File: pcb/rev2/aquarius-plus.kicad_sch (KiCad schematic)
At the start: 216 parts, among them J1 Cassette in, J10 Audio out, J11 Hand controller 2, J12 ESP USB Host, J13 Power in, J14 FPGA spare, J15 Expansion port, J16 ESP32 spare, J2 Cassette out, J3 Amphenol GSD090012SEU, J4 Printer, J5 Hand controller 1, J6 VGA, J7 DBG, J8 USB_A, J9 USB_A, Q1 BC847C, Q2 BC847C, SW1 SW_DPDT_x2, U1 XC3S200-4TQG144, U10 IS61C5128AS-25QLI, U11 74LVC4245APW, U12 74HC166, U13 SST39SF020A-55-4C-WHE, U14 74LVC4245APW, U15 LDL1117S33R, U16 MCP1700T-2502E/TT, U17 LD1117S12, U2 SN74CBTD3861PWR, U3 MAX3221ECPWR, U4 SN74CBTD3861PWR, U5 ESP32-S2-SOLO-N4R2, U6 SN74CBTD3861PWR, U7 Z84C0010AEG, U8 SN74CBTD3861PWR, U9 74HC166, X1 ECS-5032MV-143-CN-TR, X2 ECS-5032MV-480-BN-TR

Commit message: Working on rev2 PCB.
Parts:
- removed C47, C53: 100uF, Capacitor_SMD:CP_Elec_6.3x7.7, symbol Device:C_Polarized_Small
- removed C52, C56, C57, C58, C59, C60: 100nF, Capacitor_SMD:C_0603_1608Metric, symbol Device:C_Small
- removed C63, C66: 4.7uF, Capacitor_SMD:C_0603_1608Metric, symbol Device:C_Small
- removed J8, J9: USB_A, Connector_USB:USB_A_Molex_67643_Horizontal, symbol Connector:USB_A
- removed R10: DNP, Resistor_SMD:R_0603_1608Metric, symbol Device:R
- removed R100: 1, Resistor_SMD:R_0603_1608Metric, symbol Device:R
- removed R11, R2, R5, R6, R63, R64, R65, R66, R67, R68, R69, R70, R8, R91, R92, R93, R94, R95, R96, R97, R98: 4.7k, Resistor_SMD:R_0603_1608Metric, symbol Device:R
- removed R3, R4, R9: 220, Resistor_SMD:R_0603_1608Metric, symbol Device:R
- removed R7: 1k, Resistor_SMD:R_0603_1608Metric, symbol Device:R
- removed R73, R74, R75, R76: 33, Resistor_SMD:R_0603_1608Metric, symbol Device:R
- removed R77, R78, R79, R80: 15k, Resistor_SMD:R_0603_1608Metric, symbol Device:R
- removed U1: XC3S200-4TQG144, Package_QFP:TQFP-144_20x20mm_P0.5mm, symbol aquarius-plus:XC3S200-4TQG144
- removed U11, U14: 74LVC4245APW, Package_SO:TSSOP-24_4.4x7.8mm_P0.65mm, symbol Logic_LevelTranslator:SN74AVC8T245PW
- removed U12, U9: 74HC166, Package_SO:SOIC-16_3.9x9.9mm_P1.27mm, symbol 74xx:74LS166
- removed U13: SST39SF020A-55-4C-WHE, Package_SO:TSOP-I-32_12.4x8mm_P0.5mm, symbol aquarius-plus:SST39SF020A-55-4C-WHE
- removed U16: MCP1700T-2502E/TT, Package_TO_SOT_SMD:SOT-23, symbol Regulator_Linear:MCP1700-2502E_SOT23
- removed U2, U4, U6, U8: SN74CBTD3861PWR, Package_SO:TSSOP-24_4.4x7.8mm_P0.65mm, symbol 74xx:74CBTLV3861
- removed U5: ESP32-S2-SOLO-N4R2, aquarius-plus:ESP32-S2-SOLO-N4R2, symbol aquarius-plus:ESP32-S2-SOLO-N4R2
- removed X2: ECS-5032MV-480-BN-TR, Oscillator:Oscillator_SMD_SeikoEpson_SG8002LB-4Pin_5.0x3.2mm, symbol Oscillator:SG-5032CAN
- added C47: 100nF, Capacitor_SMD:C_0603_1608Metric, symbol Device:C_Small
- added Q3: 2N7002, Package_TO_SOT_SMD:SOT-23, symbol Transistor_FET:2N7002
- added R53: 220, Resistor_SMD:R_0603_1608Metric, symbol Device:R
- added U1: XC6SLX9-2TQG144C, Package_QFP:TQFP-144_20x20mm_P0.5mm, symbol aquarius-plus:XC6SLX9-2TQG144C
- added U11, U2, U4, U6: SN74CB3T3245PWR, Package_SO:TSSOP-20_4.4x6.5mm_P0.65mm, symbol aquarius-plus:SN74CB3T3245PWR
- added U5: ESP32-S3-WROOM-1-N4R2, aquarius-plus:ESP32-S2-SOLO-N4R2, symbol aquarius-plus:ESP32-S3-WROOM-1-N4R2
- added U8, U9: SN74AHCT1G125DBVR, Package_TO_SOT_SMD:SOT-23-5, symbol 74xGxx:74AHCT1G125
- J3: value Amphenol GSD090012SEU -> TF-03A; footprint Connector_Card:SD_TE_2041021 -> aquarius-plus:TF-03A
- R1: value 4.7k -> 10k
- X1: value ECS-5032MV-143-CN-TR -> SX3M14.31818M20F30TNN; footprint Oscillator:Oscillator_SMD_SeikoEpson_SG8002LB-4Pin_5.0x3.2mm -> Oscillator:Oscillator_SMD_SeikoEpson_SG8002CE-4Pin_3.2x2.5mm
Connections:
- net +2V5 is gone; now on net +3V3: C12.1, C17.1, C2.1, C22.1, C26.1, C7.1, R1.2
- net DE0 is gone; now on net D0: J15.26 (Pin_26)
- net DE1 is gone; now on net D1: J15.27 (Pin_27)
- net DE2 is gone; now on net D2: J15.28 (Pin_28)
- net DE3 is gone; now on net D3: J15.29 (Pin_29)
- net DE4 is gone; now on net D4: J15.30 (Pin_30)
- net DE5 is gone; now on net D5: J15.31 (Pin_31)
- net DE6 is gone; now on net D6: J15.32 (Pin_32)
- net DE7 is gone; now on net D7: J15.33 (Pin_33)
- net +1V2: now also C30.1, U1.128 (VCCINT), U1.19 (VCCINT), U1.28 (VCCINT), U1.52 (VCCINT), U1.89 (VCCINT)
- net +3V3: now also C35.1, C42.1, C43.1, C47.1, U1.103 (VCCO_1), U1.122 (VCCO_0), U1.125 (VCCO_0), U1.129 (VCCAUX), U1.135 (VCCO_0), U1.18 (VCCO_3), U1.20 (VCCAUX), U1.31 (VCCO_3), U1.36 (VCCAUX), U1.4 (VCCO_3), U1.42 (VCCO_2), U1.53 (VCCAUX), U1.60 (B2_IO_M1), U1.63 (VCCO_2), U1.69 (B2_IO_M0), U1.76 (VCCO_1), U1.86 (VCCO_1), U1.90 (VCCAUX), U11.20 (VCC), U2.20 (VCC), U4.20 (VCC), U5.2 (3V3), U6.20 (VCC); no longer C30.1, C51.1
- net +5V: now also C51.1, U8.5 (VCC), U9.5 (VCC); no longer C35.1, C42.1, C43.1
- net A0: now also U11.18 (B1)
- net A1: now also U11.17 (B2)
- net A10: now also U2.16 (B3)
- net A11: now also U2.15 (B4)
- net A12: now also U2.14 (B5)
- net A13: now also U2.13 (B6)
- net A14: now also U2.12 (B7)
- net A15: now also U2.11 (B8)
- net A2: now also U11.16 (B3)
- net A3: now also U11.15 (B4)
- net A4: now also U11.14 (B5)
- net A5: now also U11.13 (B6)
- net A6: now also U11.12 (B7)
- net A7: now also U11.11 (B8)
- net A8: now also U2.18 (B1)
- net A9: now also U2.17 (B2)
- net AUDIO_L: now also U1.22 (B3_IO_GCLK25)
- net AUDIO_R: now also U1.21 (B3_IO_GCLK24)
- net BA14: now also U1.143 (B0_IO_VREF)
- net BA15: now also U1.142 (B0_IO)
- net BA16: now also U1.141 (B0_IO)
- net BA17: now also U1.140 (B0_IO)
- net BA18: now also U1.139 (B0_IO)
- net BUSACK#: now also U6.11 (B8)
- net BUSREQ#: now also U6.12 (B7)
- net CART_CE#: now also U9.4
- net CASSETTE_IN: now also U1.24 (B3_IO_GCLK27)
- net CASSETTE_OUT: now also U1.23 (B3_IO_GCLK26)
- net D0: now also U4.18 (B1)
- net D1: now also U4.17 (B2)
- net D2: now also U4.16 (B3)
- net D3: now also U4.15 (B4)
- net D4: now also U4.14 (B5)
- net D5: now also U4.13 (B6)
- net D6: now also U4.12 (B7)
- net D7: now also U4.11 (B8)
- net ESP_CTS: now also U1.29 (B3_IO), U5.24 (IO47)
- net ESP_EXP0: now also U5.39 (IO1)
- net ESP_EXP1: now also U5.38 (IO2)
- net ESP_EXP2: now also U5.35 (IO42)
- net ESP_EXP3: now also U5.34 (IO41)
- net ESP_EXP4: now also U5.33 (IO40)
- net ESP_EXP5: now also U5.32 (IO39)
- net ESP_EXP6: now also U5.31 (IO38)
- net ESP_EXP7: now also U5.30 (IO37)
- net ESP_NOTIFY: now also U1.34 (B3_IO_VREF), U5.20 (IO12)
- net ESP_RTS: now also U1.32 (B3_IO), U5.22 (IO14)
- net ESP_RX: now also U1.30 (B3_IO), U5.23 (IO21)
- net ESP_TX: now also U1.33 (B3_IO), U5.21 (IO13)
- net ESP_USB_DM: now also U5.13 (IO19/USB_DM)
- net ESP_USB_DP: now also U5.14 (IO20/USB_DP)
- net FPGA_A0: now also U1.138 (B0_IO), U11.2 (A1)
- net FPGA_A1: now also U1.137 (B0_IO), U11.3 (A2)
- net FPGA_A10: now also U1.121 (B0_IO), U2.4 (A3)
- net FPGA_A11: now also U1.120 (B0_IO_VREF), U2.5 (A4)
- net FPGA_A12: now also U1.119 (B0_IO), U2.6 (A5)
- net FPGA_A13: now also U1.118 (B0_IO), U2.7 (A6)
- net FPGA_A14: now also U1.117 (B0_IO), U2.8 (A7)
- net FPGA_A15: now also U1.116 (B0_IO), U2.9 (A8)
- net FPGA_A2: now also U1.134 (B0_IO_GCLK19), U11.4 (A3)
- net FPGA_A3: now also U1.133 (B0_IO_GCLK18), U11.5 (A4)
- net FPGA_A4: now also U1.132 (B0_IO_GCLK17), U11.6 (A5)
- net FPGA_A5: now also U1.131 (B0_IO_GCLK16), U11.7 (A6)
- net FPGA_A6: now also U1.127 (B0_IO_GCLK15), U11.8 (A7)
- net FPGA_A7: now also U1.126 (B0_IO_GCLK14), U11.9 (A8)
- net FPGA_A8: now also U1.124 (B0_IO_GCLK13), U2.2 (A1)
- net FPGA_A9: now also U1.123 (B0_IO_GCLK12), U2.3 (A2)
- net FPGA_BUSACK#: now also U1.92 (B1_IO_GCLK8), U6.9 (A8)
- net FPGA_BUSREQ#: now also U1.93 (B1_IO_GCLK9), U6.8 (A7)
- net FPGA_CART_CE#: now also U1.88 (B1_IO_GCLK7), U9.2
- net FPGA_D0: now also U1.115 (B0_IO), U4.2 (A1)
- net FPGA_D1: now also U1.114 (B0_IO), U4.3 (A2)
- net FPGA_D2: now also U1.112 (B0_IO), U4.4 (A3)
- net FPGA_D3: now also U1.111 (B0_IO), U4.5 (A4)
- net FPGA_D4: now also U1.105 (B1_IO), U4.6 (A5)
- net FPGA_D5: now also U1.104 (B1_IO_VREF), U4.7 (A6)
- net FPGA_D6: now also U1.102 (B1_IO), U4.8 (A7)
- net FPGA_D7: now also U1.101 (B1_IO), U4.9 (A8)
- net FPGA_DONE: now also U1.71 (DONE), U5.12 (IO8)
- net FPGA_INT#: now also U1.95 (B1_IO_GCLK11), U6.6 (A5)
- net FPGA_IORQ#: now also U1.99 (B1_IO), U6.3 (A2)
- net FPGA_MREQ#: now also U1.100 (B1_IO), U6.2 (A1)
- net FPGA_PHI: now also U1.87 (B1_IO_GCLK6), U8.2
- net FPGA_PROG#: now also U1.37 (PROG_B), U5.25 (IO48)
- net FPGA_RD#: now also U1.98 (B1_IO), U6.4 (A3)
- net FPGA_RESET#: now also U1.94 (B1_IO_GCLK10), U6.7 (A6)
- net FPGA_WR#: now also U1.97 (B1_IO), U6.5 (A4)
- net GND: now also C47.2, Q3.2 (S), U1.108 (GND), U1.113 (GND), U1.13 (GND), U1.130 (GND), U1.136 (GND), U1.25 (GND), U1.3 (GND), U1.49 (GND), U1.54 (GND), U1.68 (GND), U1.73 (SUSPEND), U1.77 (GND), U1.91 (GND), U1.96 (GND), U11.10 (GND), U11.19 (~{OE}), U2.10 (GND), U2.19 (~{OE}), U4.10 (GND), U4.19 (~{OE}), U5.1 (GND), U5.40 (GND), U5.41 (EPAD), U6.10 (GND), U6.19 (~{OE}), U8.1, U8.3 (GND), U9.1, U9.3 (GND)
- net INT#: now also U6.14 (B5)
- net IORQ#: now also U6.17 (B2)
- net MREQ#: now also U6.18 (B1)
- net PHI: now also U8.4
- net PRINTER_IN: now also U1.26 (B3_IO)
- net PRINTER_OUT: now also U1.27 (B3_IO)
- net RAM_CE#: now also U1.85 (B1_IO_GCLK5)
- net RD#: now also U6.16 (B3)
- net RESET#: now also U6.13 (B6)
- net SD_ACTIVITY: now also U5.4 (IO4)
- net SD_MISO: now also U5.7 (IO7)
- net SD_MOSI: now also U5.9 (IO16)
- net SD_SCK: now also U5.8 (IO15)
- net SD_SSEL#: now also U5.10 (IO17)
- net SD_WP#: now also Q3.3 (D), U5.5 (IO5); no longer J3.11 (WRITE_PROTECT)
- net SPI_CS#: now also U1.74 (B2_IO_DOUT), U5.19 (IO11)
- net SPI_MISO: now also U1.39 (B2_IO_INIT_B), U5.15 (IO3)
- net SPI_MOSI: now also U1.65 (B2_IO_DIN), U5.17 (IO9)
- net SPI_SCLK: now also R53.1, U5.18 (IO10)
- net SYSCLK: now also U1.84 (B1_IO_GCLK4)
- net VGA_B0: now also U1.5 (B3_IO)
- net VGA_B1: now also U1.6 (B3_IO)
- net VGA_B2: now also U1.7 (B3_IO)
- net VGA_B3: now also U1.8 (B3_IO)
- net VGA_G0: now also U1.9 (B3_IO)
- net VGA_G1: now also U1.10 (B3_IO)
- net VGA_G2: now also U1.11 (B3_IO)
- net VGA_G3: now also U1.12 (B3_IO)
- net VGA_HSYNC: now also U1.1 (B3_IO)
- net VGA_R0: now also U1.14 (B3_IO_GCLK20)
- net VGA_R1: now also U1.15 (B3_IO_GCLK21)
- net VGA_R2: now also U1.16 (B3_IO_GCLK22)
- net VGA_R3: now also U1.17 (B3_IO_GCLK23)
- net VGA_VSYNC: now also U1.2 (B3_IO)
- net WR#: now also U6.15 (B4)
- net HC2_D02: now reaches R86.2
- net HC2_D06: now reaches R87.2
- net at R1.1: now also J3.11 (WRITE_PROTECT), Q3.1 (G)
- net HC1_D07: now reaches R61.2
- net at JP1.1 (A): now also U5.27 (IO0)
- net at C36.1, R27.2: now also U5.3 (EN)
- net at J7.2 (Pin_2): now also U5.36 (IO44/RXD0)
- net at J7.1 (Pin_1): now also U5.37 (IO43/TXD0)
- net HC1_D03: now reaches R56.2
- net HC1_D05: now reaches R57.2
- net HC1_D01: now reaches R60.2
- net HC2_D05: now reaches R85.2
- net HC1_D04: now reaches R55.2
- net HC1_D00: now reaches R62.2
- net HC1_D06: now reaches R59.2
- net HC2_D01: now reaches R88.2
- net HC2_D00: now reaches R90.2
- net HC2_D04: now reaches R83.2
- net HC2_D03: now reaches R84.2
- net HC1_D02: now reaches R58.2
- net HC2_D07: now reaches R89.2
- net RAM_ROM_WE# renamed RAM_WE#
- net RAM_WE#: now also U1.83 (B1_IO)
- net SD_CD# renamed SD_CD
- net SD_CD: now also U5.6 (IO6)
- new net: R53.2, U1.70 (B2_IO_CCLK)
- no-connect marks 21 -> 20
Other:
- note removed: "256KB Flash"
- note removed: "USB clock (48MHz)"
- note removed: "USB host via FPGA"
- moved on the sheet: C1, C10, C11, C12, C13, C14, C15, C16, C17, C18, C19, C2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

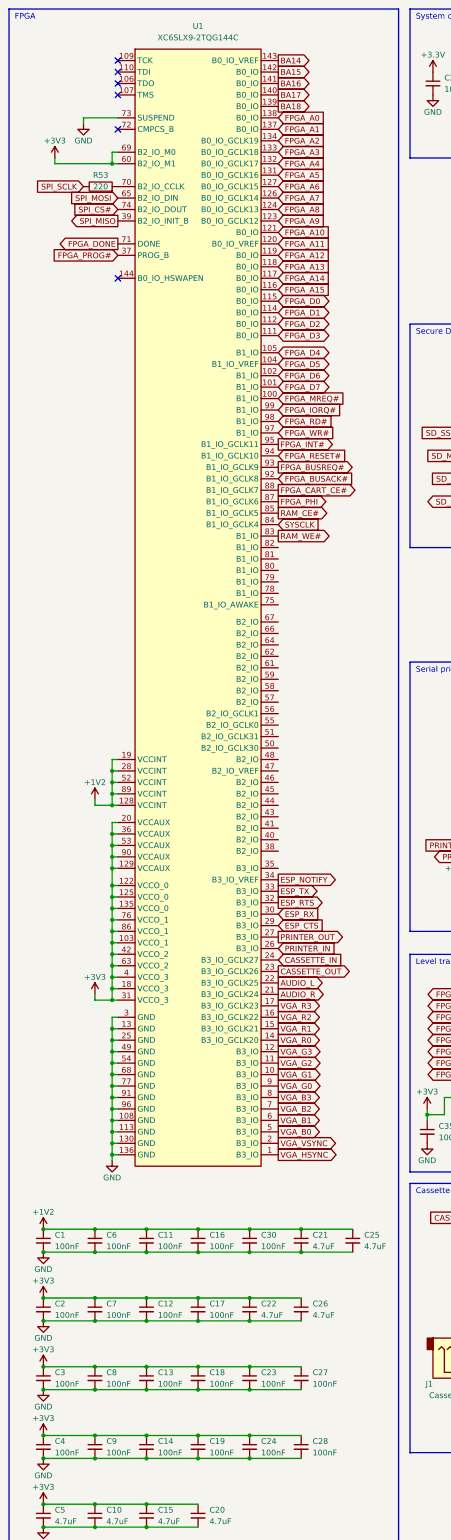
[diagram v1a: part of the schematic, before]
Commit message: A little work on rev2
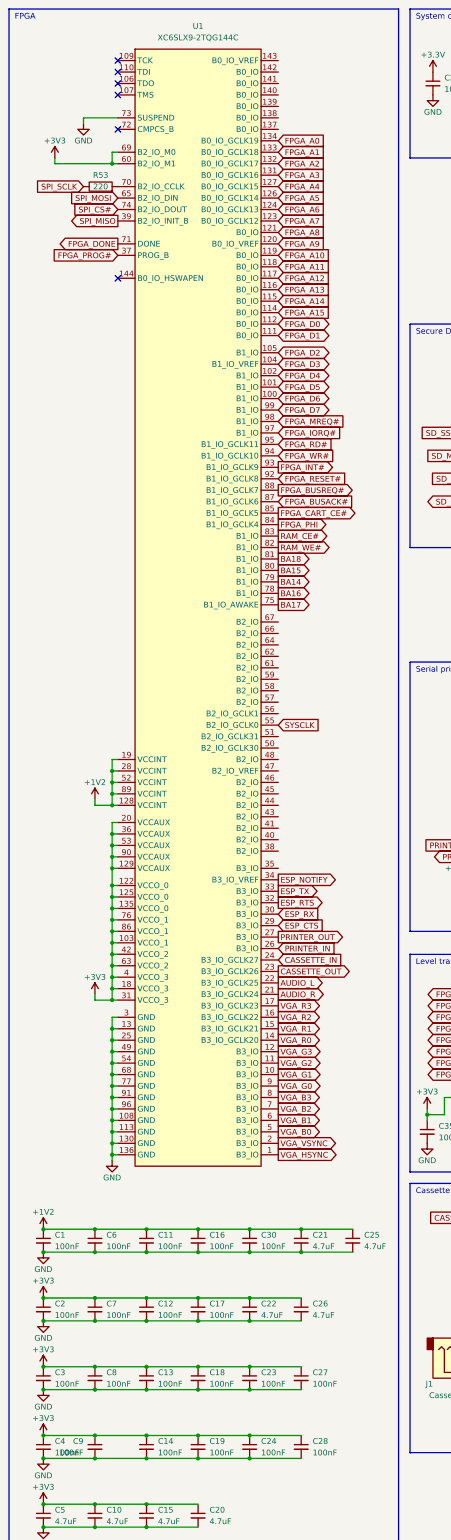
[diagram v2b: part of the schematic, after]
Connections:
- net BA14: now also U1.79 (B1_IO); no longer U1.143 (B0_IO_VREF)
- net BA15: now also U1.80 (B1_IO); no longer U1.142 (B0_IO)
- net BA16: now also U1.78 (B1_IO); no longer U1.141 (B0_IO)
- net BA17: now also U1.75 (B1_IO_AWAKE); no longer U1.140 (B0_IO)
- net BA18: now also U1.81 (B1_IO); no longer U1.139 (B0_IO)
- net FPGA_A0: now also U1.134 (B0_IO_GCLK19); no longer U1.138 (B0_IO)
- net FPGA_A1: now also U1.133 (B0_IO_GCLK18); no longer U1.137 (B0_IO)
- net FPGA_A10: now also U1.119 (B0_IO); no longer U1.121 (B0_IO)
- net FPGA_A11: now also U1.118 (B0_IO); no longer U1.120 (B0_IO_VREF)
- net FPGA_A12: now also U1.117 (B0_IO); no longer U1.119 (B0_IO)
- net FPGA_A13: now also U1.116 (B0_IO); no longer U1.118 (B0_IO)
- net FPGA_A14: now also U1.115 (B0_IO); no longer U1.117 (B0_IO)
- net FPGA_A15: now also U1.114 (B0_IO); no longer U1.116 (B0_IO)
- net FPGA_A2: now also U1.132 (B0_IO_GCLK17); no longer U1.134 (B0_IO_GCLK19)
- net FPGA_A3: now also U1.131 (B0_IO_GCLK16); no longer U1.133 (B0_IO_GCLK18)
- net FPGA_A4: now also U1.127 (B0_IO_GCLK15); no longer U1.132 (B0_IO_GCLK17)
- net FPGA_A5: now also U1.126 (B0_IO_GCLK14); no longer U1.131 (B0_IO_GCLK16)
- net FPGA_A6: now also U1.124 (B0_IO_GCLK13); no longer U1.127 (B0_IO_GCLK15)
- net FPGA_A7: now also U1.123 (B0_IO_GCLK12); no longer U1.126 (B0_IO_GCLK14)
- net FPGA_A8: now also U1.121 (B0_IO); no longer U1.124 (B0_IO_GCLK13)
- net FPGA_A9: now also U1.120 (B0_IO_VREF); no longer U1.123 (B0_IO_GCLK12)
- net FPGA_BUSACK#: now also U1.87 (B1_IO_GCLK6); no longer U1.92 (B1_IO_GCLK8)
- net FPGA_BUSREQ#: now also U1.88 (B1_IO_GCLK7); no longer U1.93 (B1_IO_GCLK9)
- net FPGA_CART_CE#: now also U1.85 (B1_IO_GCLK5); no longer U1.88 (B1_IO_GCLK7)
- net FPGA_D0: now also U1.112 (B0_IO); no longer U1.115 (B0_IO)
- net FPGA_D1: now also U1.111 (B0_IO); no longer U1.114 (B0_IO)
- net FPGA_D2: now also U1.105 (B1_IO); no longer U1.112 (B0_IO)
- net FPGA_D3: now also U1.104 (B1_IO_VREF); no longer U1.111 (B0_IO)
- net FPGA_D4: now also U1.102 (B1_IO); no longer U1.105 (B1_IO)
- net FPGA_D5: now also U1.101 (B1_IO); no longer U1.104 (B1_IO_VREF)
- net FPGA_D6: now also U1.100 (B1_IO); no longer U1.102 (B1_IO)
- net FPGA_D7: now also U1.99 (B1_IO); no longer U1.101 (B1_IO)
- net FPGA_INT#: now also U1.93 (B1_IO_GCLK9); no longer U1.95 (B1_IO_GCLK11)
- net FPGA_IORQ#: now also U1.97 (B1_IO); no longer U1.99 (B1_IO)
- net FPGA_MREQ#: now also U1.98 (B1_IO); no longer U1.100 (B1_IO)
- net FPGA_PHI: now also U1.84 (B1_IO_GCLK4); no longer U1.87 (B1_IO_GCLK6)
- net FPGA_RD#: now also U1.95 (B1_IO_GCLK11); no longer U1.98 (B1_IO)
- net FPGA_RESET#: now also U1.92 (B1_IO_GCLK8); no longer U1.94 (B1_IO_GCLK10)
- net FPGA_WR#: now also U1.94 (B1_IO_GCLK10); no longer U1.97 (B1_IO)
- net RAM_CE#: now also U1.83 (B1_IO); no longer U1.85 (B1_IO_GCLK5)
- net RAM_WE#: now also U1.82 (B1_IO); no longer U1.83 (B1_IO)
- net SYSCLK: now also U1.55 (B2_IO_GCLK0); no longer U1.84 (B1_IO_GCLK4)
